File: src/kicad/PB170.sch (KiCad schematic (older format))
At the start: 48 parts, among them J2 USB_B_Micro, Q1 BC817, Q2 BC817, Q3 BC817, Q4 BC817, SW1 SW_MEC_5E, U1 74HC08, U5 74LS73, U7 74LS73

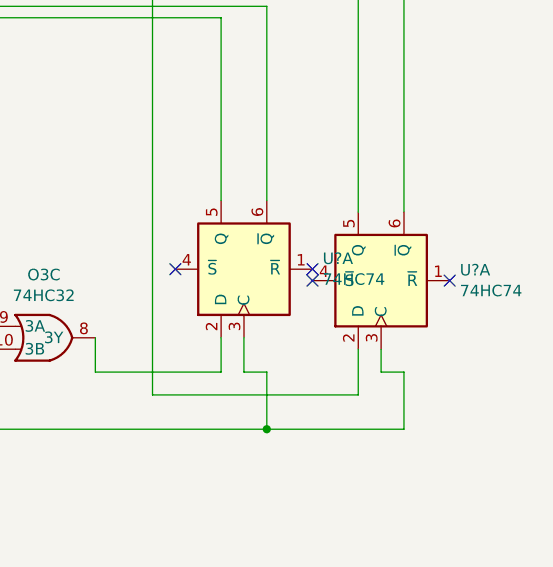
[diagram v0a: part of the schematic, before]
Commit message: D flops edit
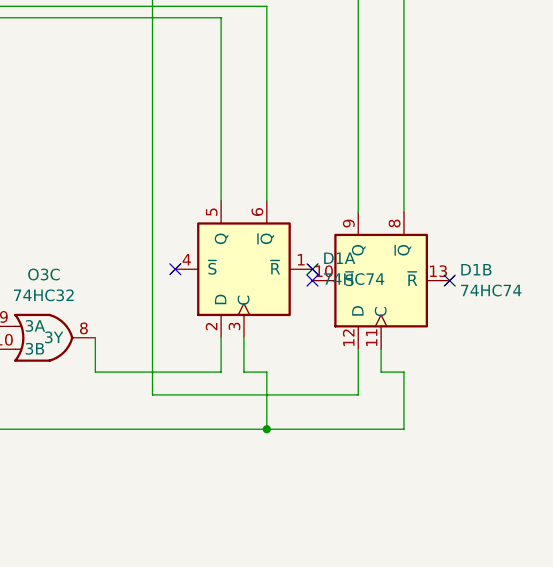
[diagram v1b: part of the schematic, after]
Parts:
- gave numbers to parts that had none: 1
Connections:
- net D2!Q: now also D1.12 (D), D1.8 (~Q); no longer D1.2 (D), D1.6 (~Q)
- net D2Q: now also D1.9 (Q); no longer D1.5 (Q)
- net at D1.3 (C): now also D1.11 (C); no longer D1.3 (C)
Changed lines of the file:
@@
 NoConn ~ 10600 5650
 $Comp
-L 74xx:74HC74 U?
-U 1 1 601F0AD7
+L 74xx:74HC74 D1
+U 2 1 601F0AD7
 P 10900 5650
-F 0 "U?" V 10946 5306 50  0000 R CNN
+F 0 "D1" V 10946 5306 50  0000 R CNN
 F 1 "74HC74" V 10855 5306 50  0000 R CNN
 F 2 "Housings_SSOP:TSSOP-14_4.4x5mm_Pitch0.65mm" H 10900 5650 50  0001 C CNN
 F 3 "74xx/74hc_hct74.pdf" H 10900 5650 50  0001 C CNN
-	1    10900 5650
+	2    10900 5650
 	0    -1   -1   0
 $EndComp
 $Comp
-L 74xx:74HC74 U?
+L 74xx:74HC74 D1
 U 1 1 601F3650
 P 10300 5600
-F 0 "U?" V 10346 5256 50  0000 R CNN
+F 0 "D1" V 10346 5256 50  0000 R CNN
 F 1 "74HC74" V 10255 5256 50  0000 R CNN
 F 2 "Housings_SSOP:TSSOP-14_4.4x5mm_Pitch0.65mm" H 10300 5600 50  0001 C CNN
